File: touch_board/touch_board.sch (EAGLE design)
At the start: 51 parts, among them IC1 PIC18F47K42-I_PT, IC2 MAX203EEWP, K1 G6K-2P, X1 RS-232-1, X2 RS-232-2, X5 Relay conn, X6 MINI-USB-UX60A-MB-5ST

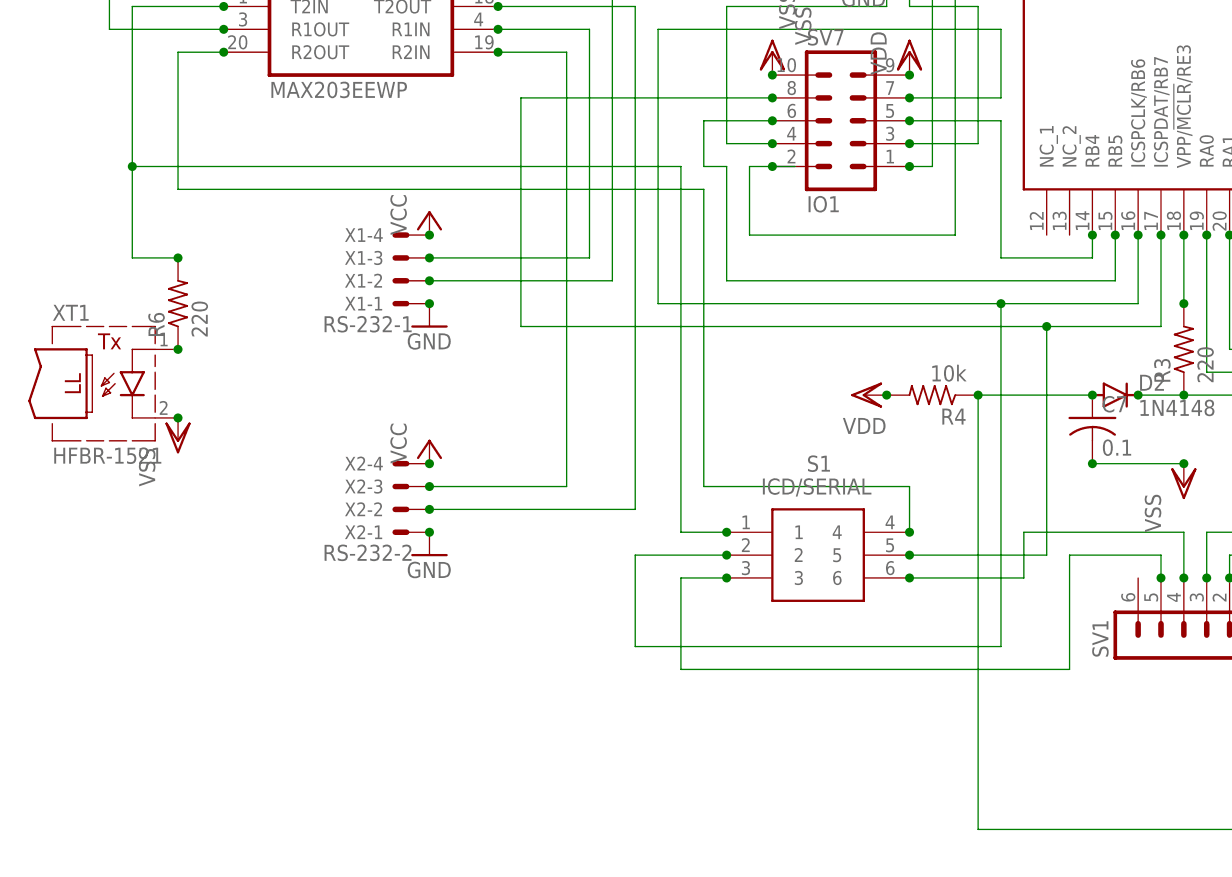
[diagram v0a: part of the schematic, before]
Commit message: update
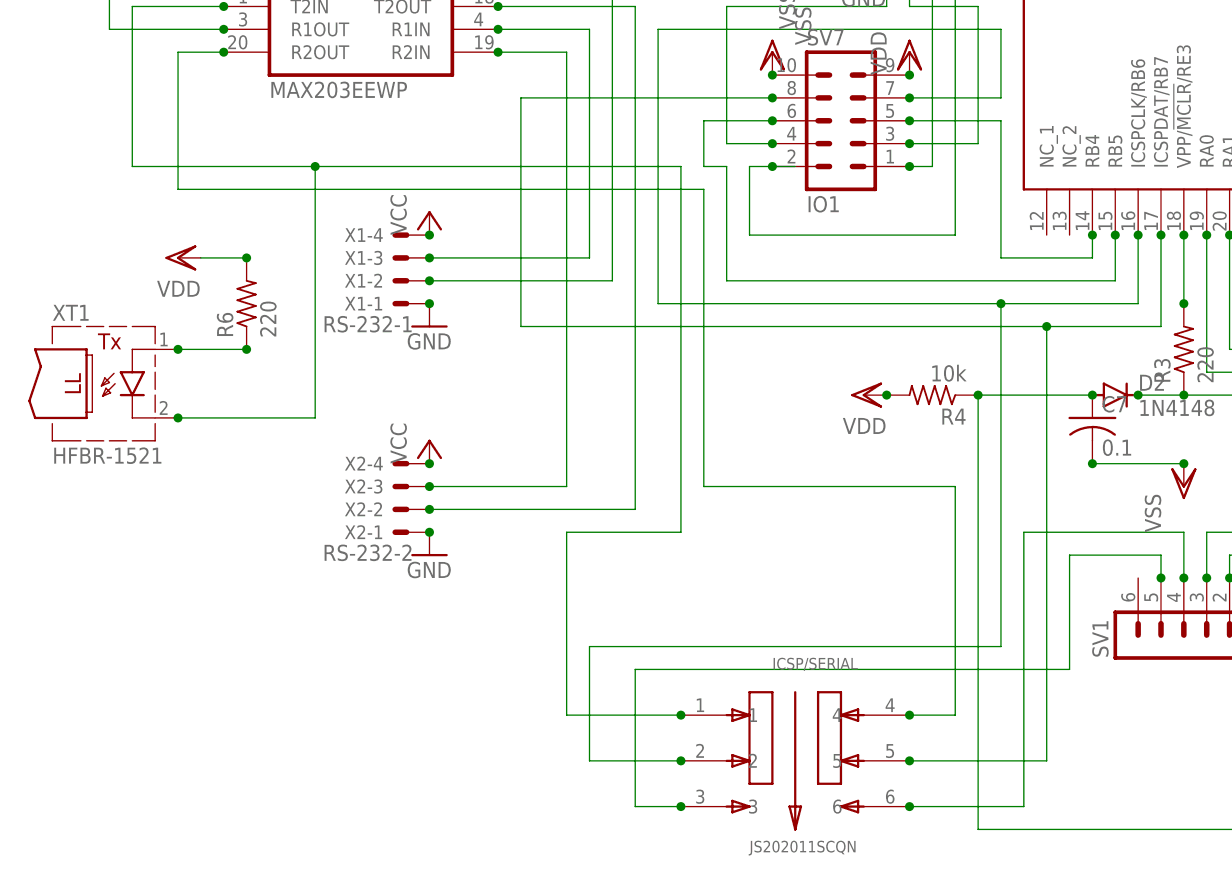
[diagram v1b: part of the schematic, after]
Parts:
- removed S1: ICD/SERIAL, JS202011SCQN:JS202011SCQN
- added ICSP/SERIAL: JS202011SCQN, JS202011SCQN_fixed:JS202011SCQN
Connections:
- net N$20: now also ICSP/SERIAL.1, XT1.C; no longer R6.2, S1.1
- net N$22: now also ICSP/SERIAL.4; no longer S1.4
- net N$23: now also ICSP/SERIAL.6; no longer S1.6
- net N$6: now also ICSP/SERIAL.5; no longer S1.5
- net N$65: now also ICSP/SERIAL.3; no longer S1.3
- net N$7: now also ICSP/SERIAL.2; no longer S1.2
- net VDD: now also R6.2
- net VSS: no longer XT1.C
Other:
- moved on the sheet: R6

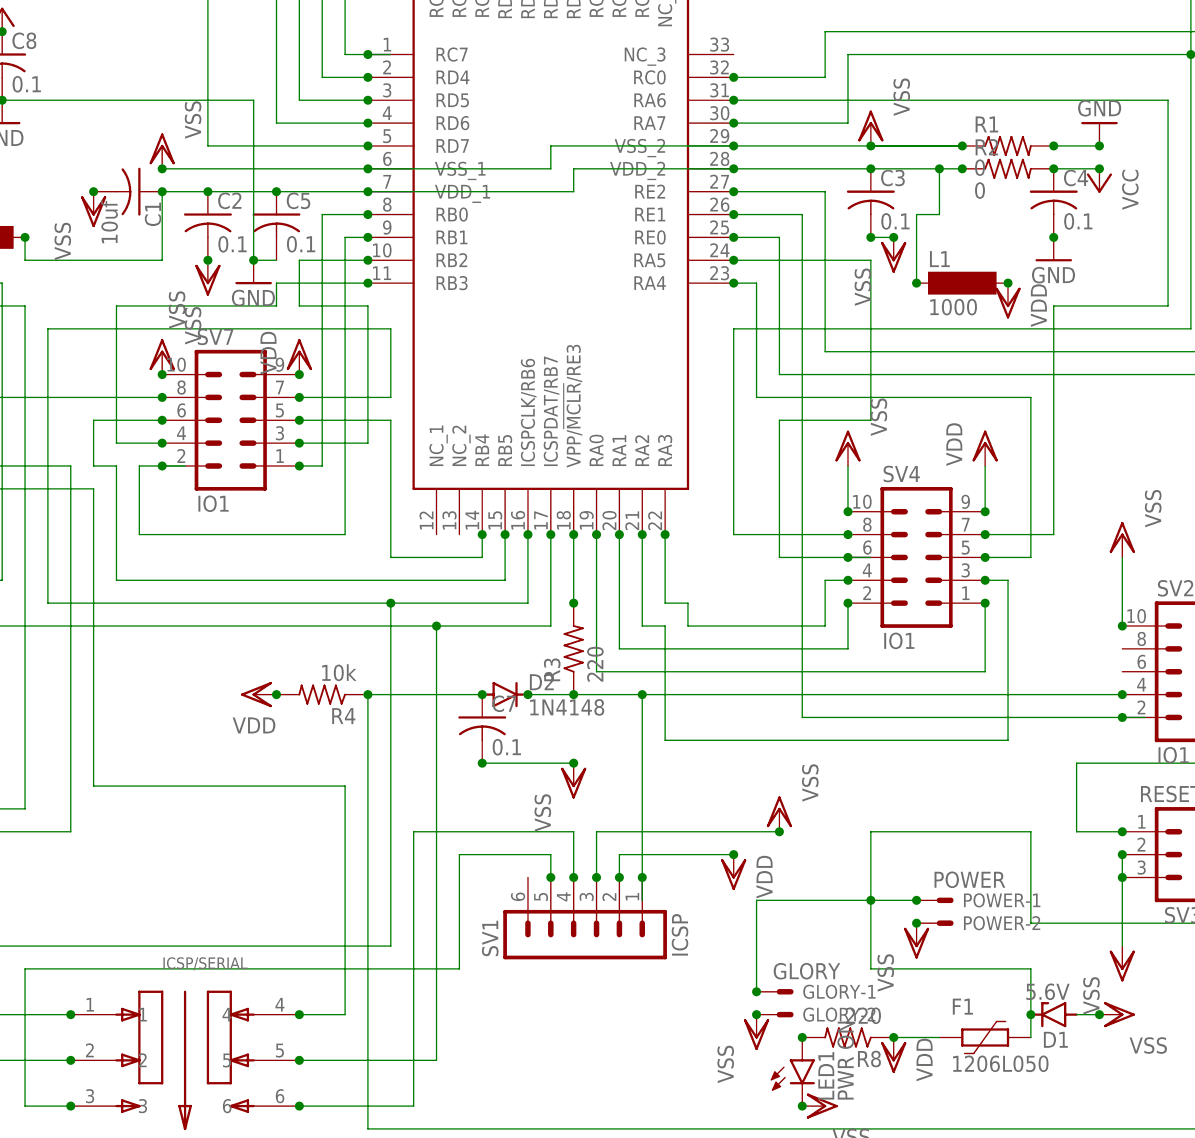
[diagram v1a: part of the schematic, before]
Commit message: update
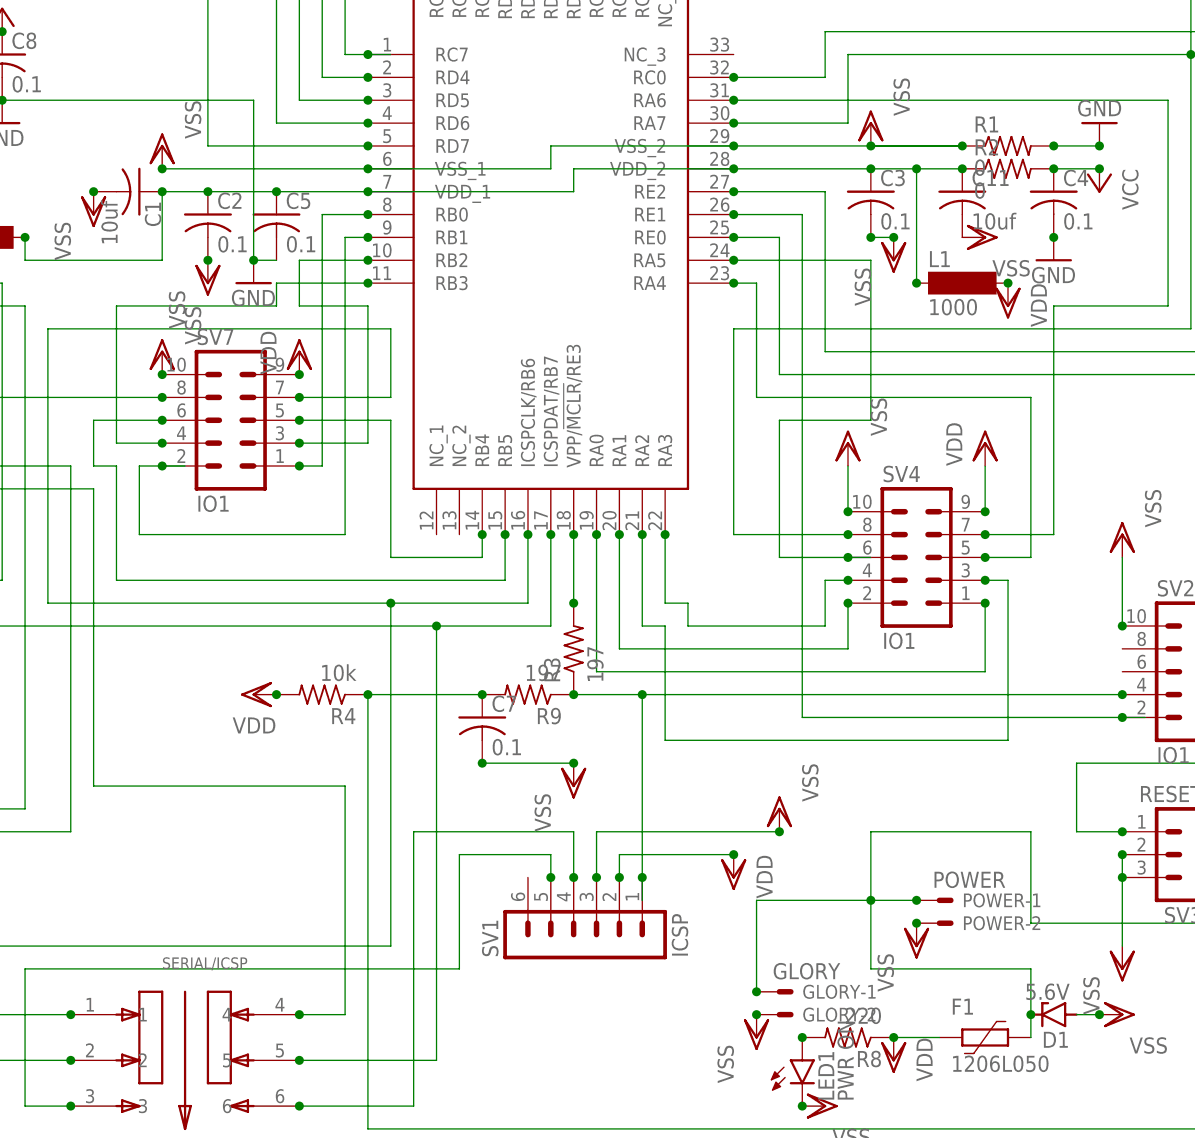
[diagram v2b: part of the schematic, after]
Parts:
- removed D2: 1N4148, diode:CGRM4001-G
- added C11: 10uf, rcl:C-USC0805
- added R9: 197, rcl:R-US_R0805
- R3: value 220 -> 197
- renumbered ICSP/SERIAL to SERIAL/ICSP
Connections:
- net N$2: now also R9.1; no longer D2.C
- net N$58: now also C11.1
- net N$62: now also R9.2; no longer D2.A
- net VSS: now also C11.2
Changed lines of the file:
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@@
 <part name="C7" library="rcl" library_urn="urn:adsk.eagle:library:334" deviceset="C-US" device="C0805" package3d_urn="urn:adsk.eagle:package:23617/2" value="0.1"/>
 <part name="VSS7" library="supply1" library_urn="urn:adsk.eagle:library:371" deviceset="VSS" device=""/>
-<part name="R3" library="rcl" library_urn="urn:adsk.eagle:library:334" deviceset="R-US_" device="R0805" package3d_urn="urn:adsk.eagle:package:23553/2" value="220"/>
+<part name="R3" library="rcl" library_urn="urn:adsk.eagle:library:334" deviceset="R-US_" device="R0805" package3d_urn="urn:adsk.eagle:package:23553/2" value="197"/>
 <part name="R4" library="rcl" library_urn="urn:adsk.eagle:library:334" deviceset="R-US_" device="R0805" package3d_urn="urn:adsk.eagle:package:23553/2" value="10k"/>
 <part name="VDD5" library="supply1" library_urn="urn:adsk.eagle:library:371" deviceset="VDD" device=""/>
@@
 <part name="VSS24" library="supply1" library_urn="urn:adsk.eagle:library:371" deviceset="VSS" device=""/>
 <part name="VSS25" library="supply1" library_urn="urn:adsk.eagle:library:371" deviceset="VSS" device=""/>
-<part name="D2" library="diode" library_urn="urn:adsk.eagle:library:210" deviceset="CGRM400*-G" device="" package3d_urn="urn:adsk.eagle:package:43457/2" technology="1" value="1N4148"/>
 <part name="SV8" library="con-lstb" library_urn="urn:adsk.eagle:library:162" deviceset="MA10-1" device="" package3d_urn="urn:adsk.eagle:package:8346/1" value="LCD"/>
 <part name="C10" library="rcl" library_urn="urn:adsk.eagle:library:334" deviceset="C-US" device="C0805" package3d_urn="urn:adsk.eagle:package:23617/2" value="0.1"/>
@@
 <part name="SV9" library="con-lstb" library_urn="urn:adsk.eagle:library:162" deviceset="MA03-1" device="" package3d_urn="urn:adsk.eagle:package:8339/1" value="USBH"/>
 <part name="X6" library="con-hirose" library_urn="urn:adsk.eagle:library:152" deviceset="MINI-USB-" device="UX60A-MB-5ST" package3d_urn="urn:adsk.eagle:package:7263/1"/>
-<part name="ICSP/SERIAL" library="JS202011SCQN_fixed" deviceset="JS202011SCQN" device=""/>
+<part name="SERIAL/ICSP" library="JS202011SCQN_fixed" deviceset="JS202011SCQN" device=""/>
 <part name="VDD8" library="supply1" library_urn="urn:adsk.eagle:library:371" deviceset="VDD" device=""/>
+<part name="R9" library="rcl" library_urn="urn:adsk.eagle:library:334" deviceset="R-US_" device="R0805" package3d_urn="urn:adsk.eagle:package:23553/2" value="197"/>
+<part name="C11" library="rcl" library_urn="urn:adsk.eagle:library:334" deviceset="C-US" device="C0805" package3d_urn="urn:adsk.eagle:package:23617/2" value="10uf"/>
+<part name="VSS15" library="supply1" library_urn="urn:adsk.eagle:library:371" deviceset="VSS" device=""/>
 </parts>
 <sheets>
@@
 <attribute name="VALUE" x="182.88" y="-66.04" size="1.778" layer="96" rot="R90"/>
 </instance>
-<instance part="D2" gate="G$1" x="68.58" y="-20.32" smashed="yes">
-<attribute name="NAME" x="71.12" y="-19.8374" size="1.778" layer="95"/>
-<attribute name="VALUE" x="71.12" y="-22.6314" size="1.778" layer="96"/>
-</instance>
 <instance part="SV8" gate="1" x="200.66" y="27.94" smashed="yes" rot="R180">
 <attribute name="VALUE" x="201.93" y="43.18" size="1.778" layer="96" rot="R180"/>
@@
 <attribute name="VALUE" x="198.12" y="-27.94" size="1.778" layer="96" rot="R90"/>
 </instance>
-<instance part="ICSP/SERIAL" gate="G$1" x="33.02" y="-60.96" smashed="yes" rot="R270">
+<instance part="SERIAL/ICSP" gate="G$1" x="33.02" y="-60.96" smashed="yes" rot="R270">
 <attribute name="NAME" x="30.4578" y="-50.7963" size="1.27185" layer="95"/>
 <attribute name="VALUE" x="27.9288" y="-71.123740625" size="1.270940625" layer="96"/>
@@
 <instance part="VDD8" gate="G$1" x="-35.56" y="-5.08" smashed="yes" rot="R90">
 <attribute name="VALUE" x="-33.02" y="-7.62" size="1.778" layer="96" rot="R180"/>
+</instance>
+<instance part="R9" gate="G$1" x="71.12" y="-20.32" smashed="yes" rot="R180">
+<attribute name="NAME" x="74.93" y="-21.8186" size="1.778" layer="95" rot="R180"/>
+<attribute name="VALUE" x="74.93" y="-17.018" size="1.778" layer="96" rot="R180"/>
+</instance>
+<instance part="C11" gate="G$1" x="119.38" y="35.56" smashed="yes">
+<attribute name="NAME" x="120.396" y="36.195" size="1.778" layer="95"/>
+<attribute name="VALUE" x="120.396" y="31.369" size="1.778" layer="96"/>
+</instance>
+<instance part="VSS15" gate="G$1" x="121.92" y="30.48" smashed="yes" rot="R90">
+<attribute name="VALUE" x="127" y="27.94" size="1.778" layer="96" rot="R180"/>
 </instance>
 </instances>
@@
 <junction x="182.88" y="-25.4"/>
 </segment>
+<segment>
+<pinref part="C11" gate="G$1" pin="2"/>
+<pinref part="VSS15" gate="G$1" pin="VSS"/>
+</segment>
 </net>
 <net name="VDD" class="0">
@@
 <junction x="83.82" y="-20.32"/>
 <junction x="137.16" y="-20.32"/>
-<pinref part="D2" gate="G$1" pin="C"/>
-<wire x1="71.12" y1="-20.32" x2="76.2" y2="-20.32" width="0.1524" layer="91"/>
-<junction x="71.12" y="-20.32"/>
+<pinref part="R9" gate="G$1" pin="1"/>
 <junction x="76.2" y="-20.32"/>
 </segment>
@@
 <junction x="60.96" y="-12.7"/>
 <junction x="30.48" y="12.7"/>
-<pinref part="ICSP/SERIAL" gate="G$1" pin="5"/>
+<pinref part="SERIAL/ICSP" gate="G$1" pin="5"/>
 <wire x1="45.72" y1="-60.96" x2="60.96" y2="-60.96" width="0.1524" layer="91"/>
 <junction x="45.72" y="-60.96"/>
@@
 <junction x="45.72" y="12.7"/>
 <junction x="55.88" y="-10.16"/>
-<pinref part="ICSP/SERIAL" gate="G$1" pin="2"/>
+<pinref part="SERIAL/ICSP" gate="G$1" pin="2"/>
 <wire x1="10.16" y1="-48.26" x2="10.16" y2="-60.96" width="0.1524" layer="91"/>
 <wire x1="10.16" y1="-60.96" x2="20.32" y2="-60.96" width="0.1524" layer="91"/>
@@
 <wire x1="20.32" y1="-35.56" x2="7.62" y2="-35.56" width="0.1524" layer="91"/>
 <wire x1="7.62" y1="-35.56" x2="7.62" y2="-55.88" width="0.1524" layer="91"/>
-<pinref part="ICSP/SERIAL" gate="G$1" pin="1"/>
+<pinref part="SERIAL/ICSP" gate="G$1" pin="1"/>
 <wire x1="7.62" y1="-55.88" x2="20.32" y2="-55.88" width="0.1524" layer="91"/>
 <junction x="20.32" y="-55.88"/>
@@
 <wire x1="22.86" y1="2.54" x2="22.86" y2="-30.48" width="0.1524" layer="91"/>
 <wire x1="22.86" y1="-30.48" x2="50.8" y2="-30.48" width="0.1524" layer="91"/>
-<pinref part="ICSP/SERIAL" gate="G$1" pin="4"/>
+<pinref part="SERIAL/ICSP" gate="G$1" pin="4"/>
 <wire x1="45.72" y1="-55.88" x2="50.8" y2="-55.88" width="0.1524" layer="91"/>
 <wire x1="50.8" y1="-55.88" x2="50.8" y2="-30.48" width="0.1524" layer="91"/>
@@
 <wire x1="58.42" y1="-35.56" x2="76.2" y2="-35.56" width="0.1524" layer="91"/>
 <wire x1="58.42" y1="-35.56" x2="58.42" y2="-66.04" width="0.1524" layer="91"/>
-<pinref part="ICSP/SERIAL" gate="G$1" pin="6"/>
+<pinref part="SERIAL/ICSP" gate="G$1" pin="6"/>
 <wire x1="58.42" y1="-66.04" x2="45.72" y2="-66.04" width="0.1524" layer="91"/>
 <junction x="45.72" y="-66.04"/>
@@
 <pinref part="C3" gate="G$1" pin="1"/>
 <junction x="109.22" y="38.1"/>
-<wire x1="119.38" y1="38.1" x2="116.84" y2="38.1" width="0.1524" layer="91"/>
+<wire x1="119.38" y1="38.1" x2="114.3" y2="38.1" width="0.1524" layer="91"/>
 <pinref part="C5" gate="G$1" pin="1"/>
 <junction x="43.18" y="35.56"/>
 <pinref part="L2" gate="G$1" pin="2"/>
-<wire x1="116.84" y1="38.1" x2="109.22" y2="38.1" width="0.1524" layer="91"/>
+<wire x1="114.3" y1="38.1" x2="109.22" y2="38.1" width="0.1524" layer="91"/>
 <wire x1="15.24" y1="30.48" x2="15.24" y2="27.94" width="0.1524" layer="91"/>
 <wire x1="15.24" y1="27.94" x2="30.48" y2="27.94" width="0.1524" layer="91"/>
 <wire x1="30.48" y1="27.94" x2="30.48" y2="35.56" width="0.1524" layer="91"/>
 <pinref part="L1" gate="G$1" pin="1"/>
-<wire x1="114.3" y1="25.4" x2="114.3" y2="33.02" width="0.1524" layer="91"/>
-<wire x1="114.3" y1="33.02" x2="116.84" y2="33.02" width="0.1524" layer="91"/>
-<wire x1="116.84" y1="33.02" x2="116.84" y2="38.1" width="0.1524" layer="91"/>
+<wire x1="114.3" y1="25.4" x2="114.3" y2="38.1" width="0.1524" layer="91"/>
 <junction x="15.24" y="30.48"/>
 <junction x="30.48" y="35.56"/>
 <junction x="114.3" y="25.4"/>
-<junction x="116.84" y="38.1"/>
+<junction x="114.3" y="38.1"/>
+<pinref part="C11" gate="G$1" pin="1"/>
 </segment>
 </net>
@@
 <junction x="53.34" y="-20.32"/>
 <wire x1="53.34" y1="-20.32" x2="66.04" y2="-20.32" width="0.1524" layer="91"/>
-<pinref part="D2" gate="G$1" pin="A"/>
-<junction x="66.04" y="-20.32"/>
 <wire x1="53.34" y1="-68.58" x2="53.34" y2="-20.32" width="0.1524" layer="91"/>
 <junction x="152.4" y="-50.8"/>
+<pinref part="R9" gate="G$1" pin="2"/>
+<junction x="66.04" y="-20.32"/>
 </segment>
 </net>
@@
 <wire x1="63.5" y1="-50.8" x2="15.24" y2="-50.8" width="0.1524" layer="91"/>
 <wire x1="15.24" y1="-50.8" x2="15.24" y2="-66.04" width="0.1524" layer="91"/>
-<pinref part="ICSP/SERIAL" gate="G$1" pin="3"/>
+<pinref part="SERIAL/ICSP" gate="G$1" pin="3"/>
 <wire x1="15.24" y1="-66.04" x2="20.32" y2="-66.04" width="0.1524" layer="91"/>
 <junction x="20.32" y="-66.04"/>
